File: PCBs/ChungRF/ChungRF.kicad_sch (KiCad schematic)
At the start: 15 parts, among them J1 Conn_Coaxial, J2 Conn_01x09_Socket, U1 E22-900M30S

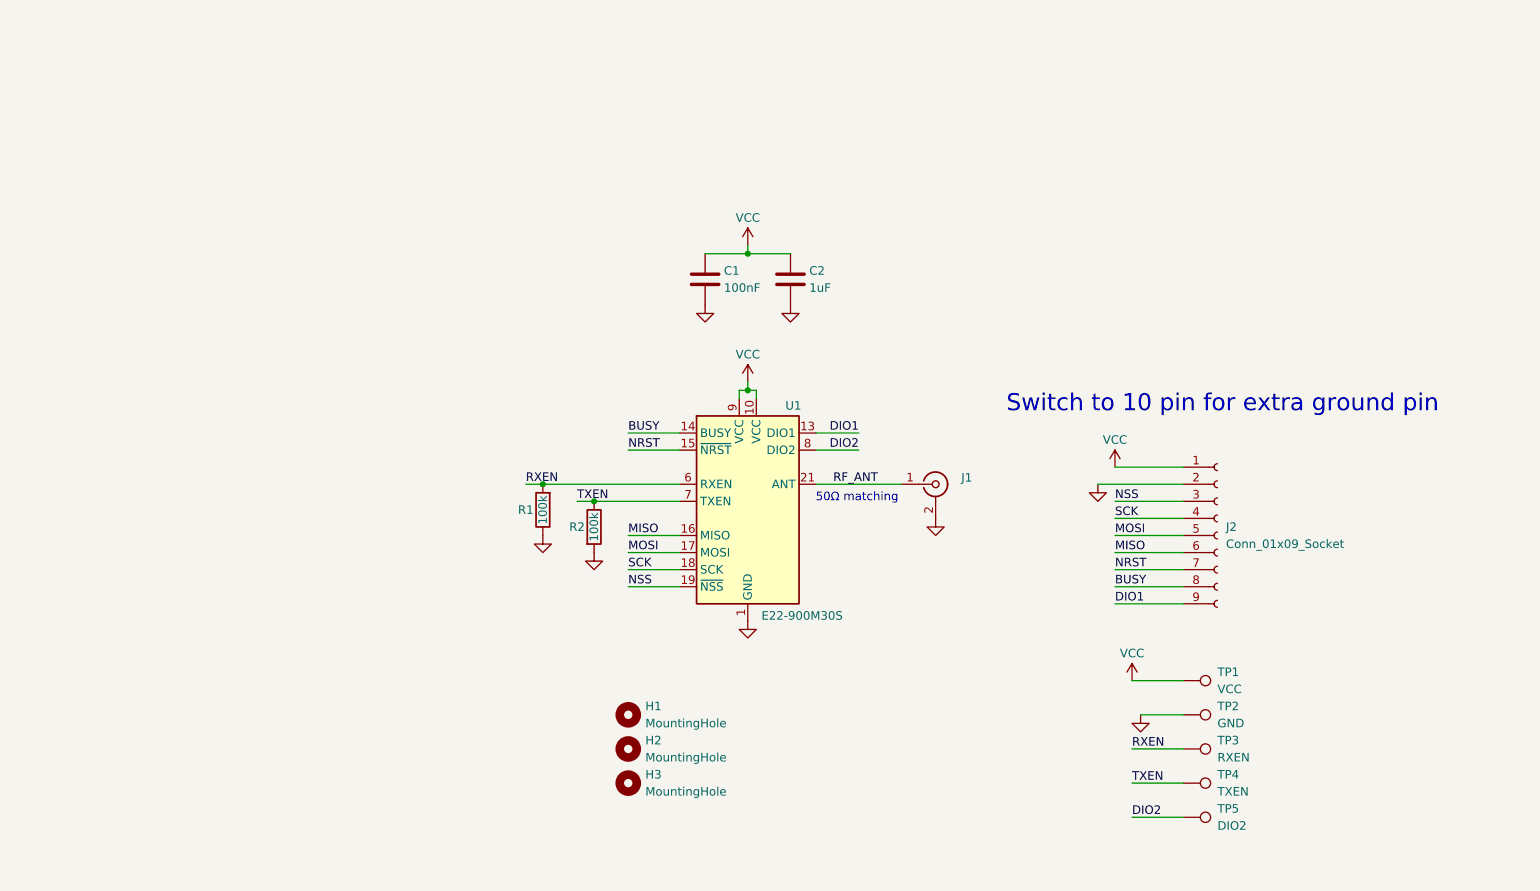
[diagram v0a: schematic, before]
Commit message: ChungRF R2
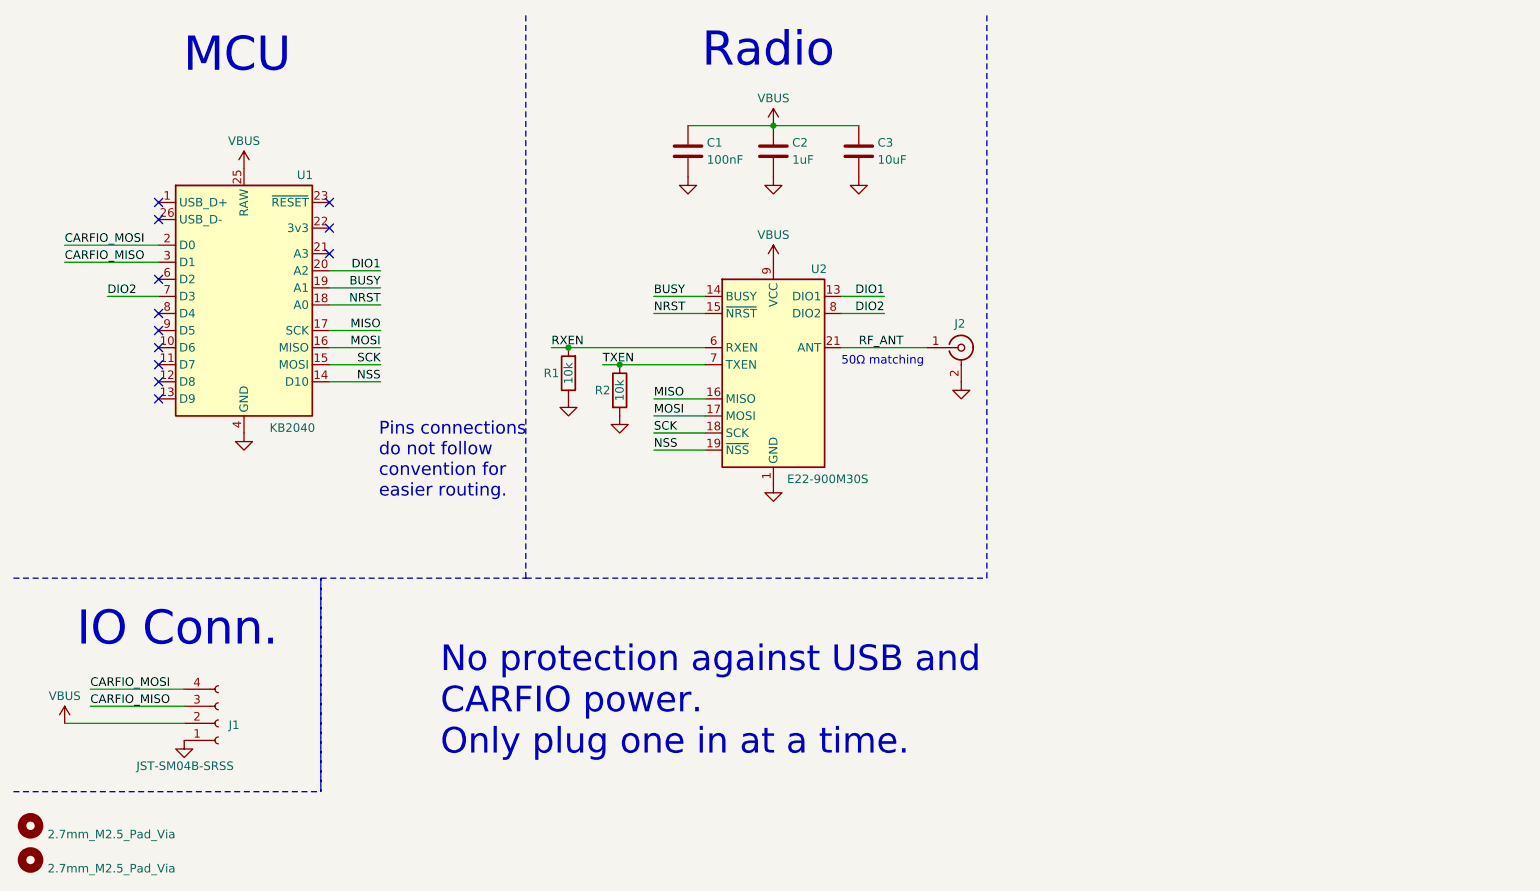
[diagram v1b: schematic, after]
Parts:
- removed H3: MountingHole, MountingHole:MountingHole_2.7mm_M2.5_Pad_Via, symbol Mechanical:MountingHole
- removed J2: Conn_01x09_Socket, Connector_JST:JST_SH_SM09B-SRSS-TB_1x09-1MP_P1.00mm_Horizontal, symbol Connector:Conn_01x09_Socket
- removed TP1: VCC, TestPoint:TestPoint_Pad_D1.5mm, symbol Connector:TestPoint
- removed TP2: GND, TestPoint:TestPoint_Pad_D1.5mm, symbol Connector:TestPoint
- removed TP3: RXEN, TestPoint:TestPoint_Pad_D1.5mm, symbol Connector:TestPoint
- removed TP4: TXEN, TestPoint:TestPoint_Pad_D1.5mm, symbol Connector:TestPoint
- removed TP5: DIO2, TestPoint:TestPoint_Pad_D1.5mm, symbol Connector:TestPoint
- added C3: 10uF, Capacitor_SMD:C_0603_1608Metric, symbol Device:C
- added J1: JST-SM04B-SRSS, besser_footprints:JST_SH_SM04B-SRSS-TB_1x04-1MP_P1.00mm_Horizontal, symbol Connector:Conn_01x04_Socket
- added U1: KB2040, besser_footprints:Adafuit-KB2040-SMD, symbol besserLib:Adafruit-KB2040
- H1, H2: value MountingHole -> 2.7mm_M2.5_Pad_Via
- J2: renamed from J1; footprint besser_footprints:CON-SMA-EDGE-S -> besser_footprints:CONSMA003.062
- R1, R2: value 100k -> 10k
- renumbered U1 to U2
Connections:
- net BUSY: now also U1.19 (A1)
- net DIO1: now also U1.20 (A2)
- net DIO2: now also U1.7 (D3)
- net GND: now also C3.2, J1.1 (Pin_1), U1.24 (GND), U1.4 (GND), U1.5 (GND)
- net MISO: now also U1.17 (SCK)
- net MOSI: now also U1.16 (MISO)
- net NRST: now also U1.18 (A0)
- net NSS: now also U1.14 (D10)
- net SCK: now also U1.15 (MOSI)
- net VCC renamed VBUS
- net VBUS: now also C3.1, J1.2 (Pin_2), U1.25 (RAW)
- new net CARFIO_MISO: J1.3 (Pin_3), U1.3 (D1)
- new net CARFIO_MOSI: J1.4 (Pin_4), U1.2 (D0)
- no-connect marks 0 -> 12
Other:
- note added: "IO Conn."
- note added: "MCU"
- note added: "No protection against USB and CARFIO power. Only plug one in at a time."
- note added: "Pins connections do not follow convention for easier routing."
- note added: "Radio"
- note removed: "Switch to 10 pin for extra ground pin"
- moved on the sheet: C1, C2, J2, R1, R2
